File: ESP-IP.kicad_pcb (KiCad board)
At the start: 2 copper layers, 32 parts, among them J1 Serial and power, J2 Programming Pads, Q1 L78M05ABDT-TR, SW1 SW_Push, SW2 SW_Push, U1 ESP32-WROOM-32U, U3 TXS0102DCU, U4 AMS1117-3.3

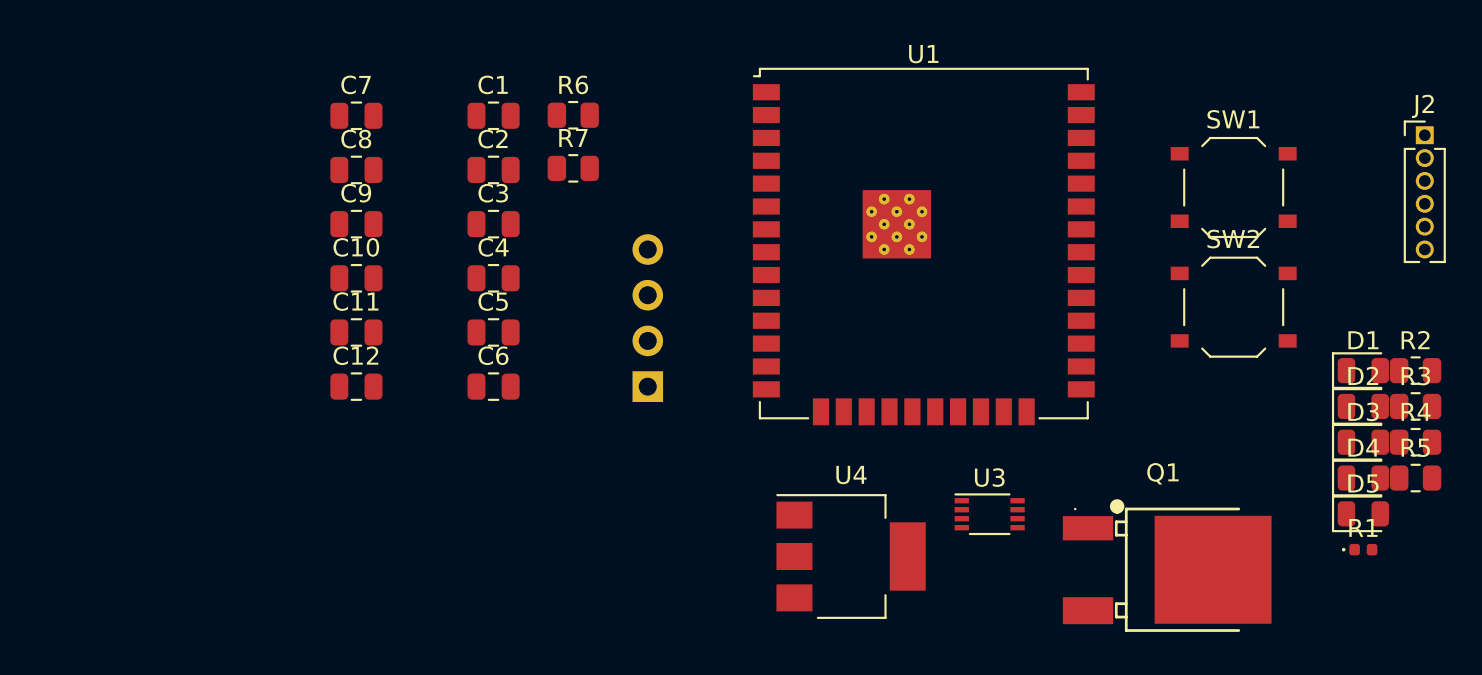
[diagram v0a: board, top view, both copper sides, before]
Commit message: feat: moving around bits and bobs
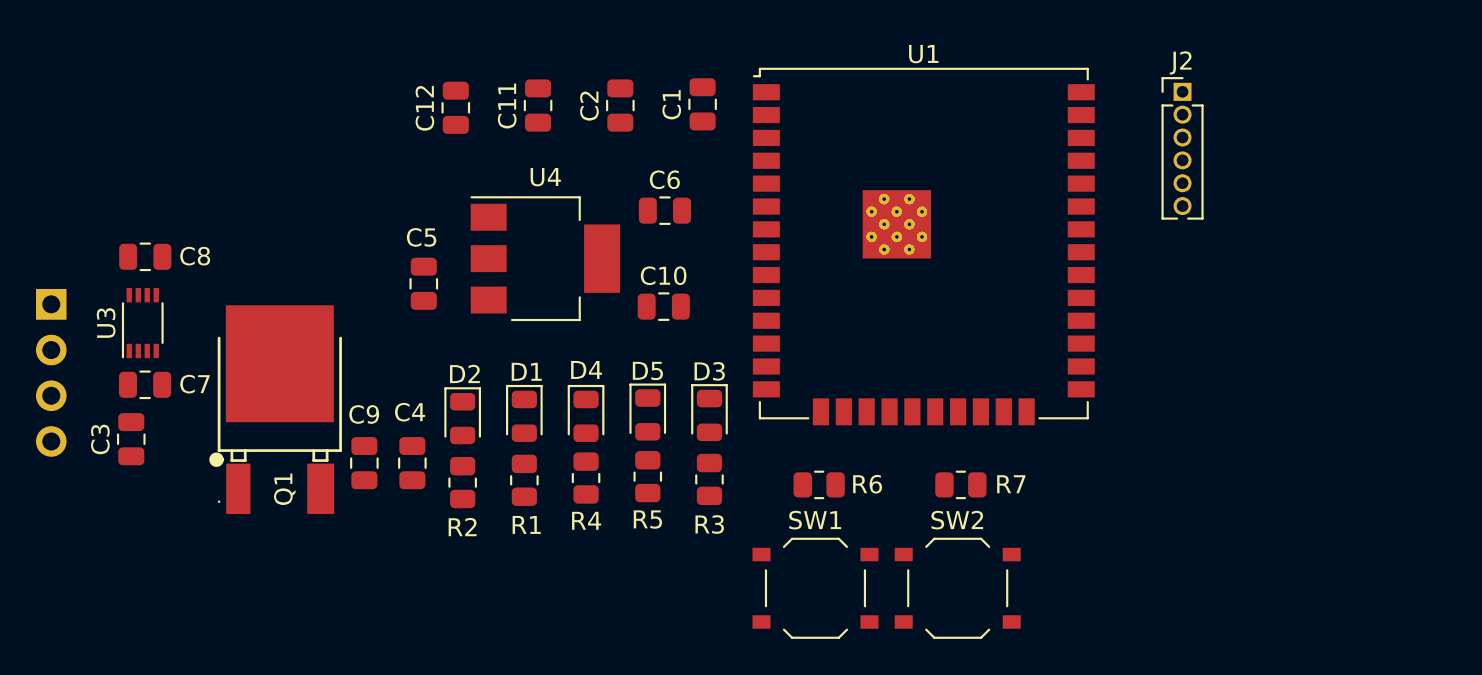
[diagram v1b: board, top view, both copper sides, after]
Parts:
- R1: footprint LED_SMD:LED_0402_1005Metric -> Resistor_SMD:R_0805_2012Metric
- moved R2 53.3 mm to (106.6, 81.5), turned to 90 degrees
- moved D2 50.1 mm to (106.6, 78.0), turned to -90 degrees
- moved Q1 49.1 mm to (96.4, 78.4), turned to 90 degrees
- moved U3 48.2 mm to (88.8, 72.7), turned to 90 degrees
- moved R1 46.8 mm to (110.0, 81.4), turned to 90 degrees
- moved D1 46.7 mm to (110.0, 77.9), turned to -90 degrees
- moved R4 46.1 mm to (113.4, 81.3), turned to 90 degrees
- moved D4 43.3 mm to (113.4, 77.9), turned to -90 degrees
- moved R5 42.7 mm to (116.8, 81.2), turned to 90 degrees
- moved D5 40.1 mm to (116.8, 77.8), turned to -90 degrees
- moved R3 39.5 mm to (120.3, 81.4), turned to 90 degrees
- moved D3 36.4 mm to (120.3, 77.8), turned to -90 degrees
- moved J1 33.5 mm to (83.7, 71.6), turned to 180 degrees
- moved SW1 32.2 mm to (126.2, 87.4)
- moved R7 27.8 mm to (134.2, 81.7), turned to 180 degrees
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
